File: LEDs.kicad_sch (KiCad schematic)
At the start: 26 parts, among them J3 JST-PH-1x3, J4 JST-PH-1x3, U4 SN74LVC1T45DBVR, U6 SN74LVC1T45DBVR

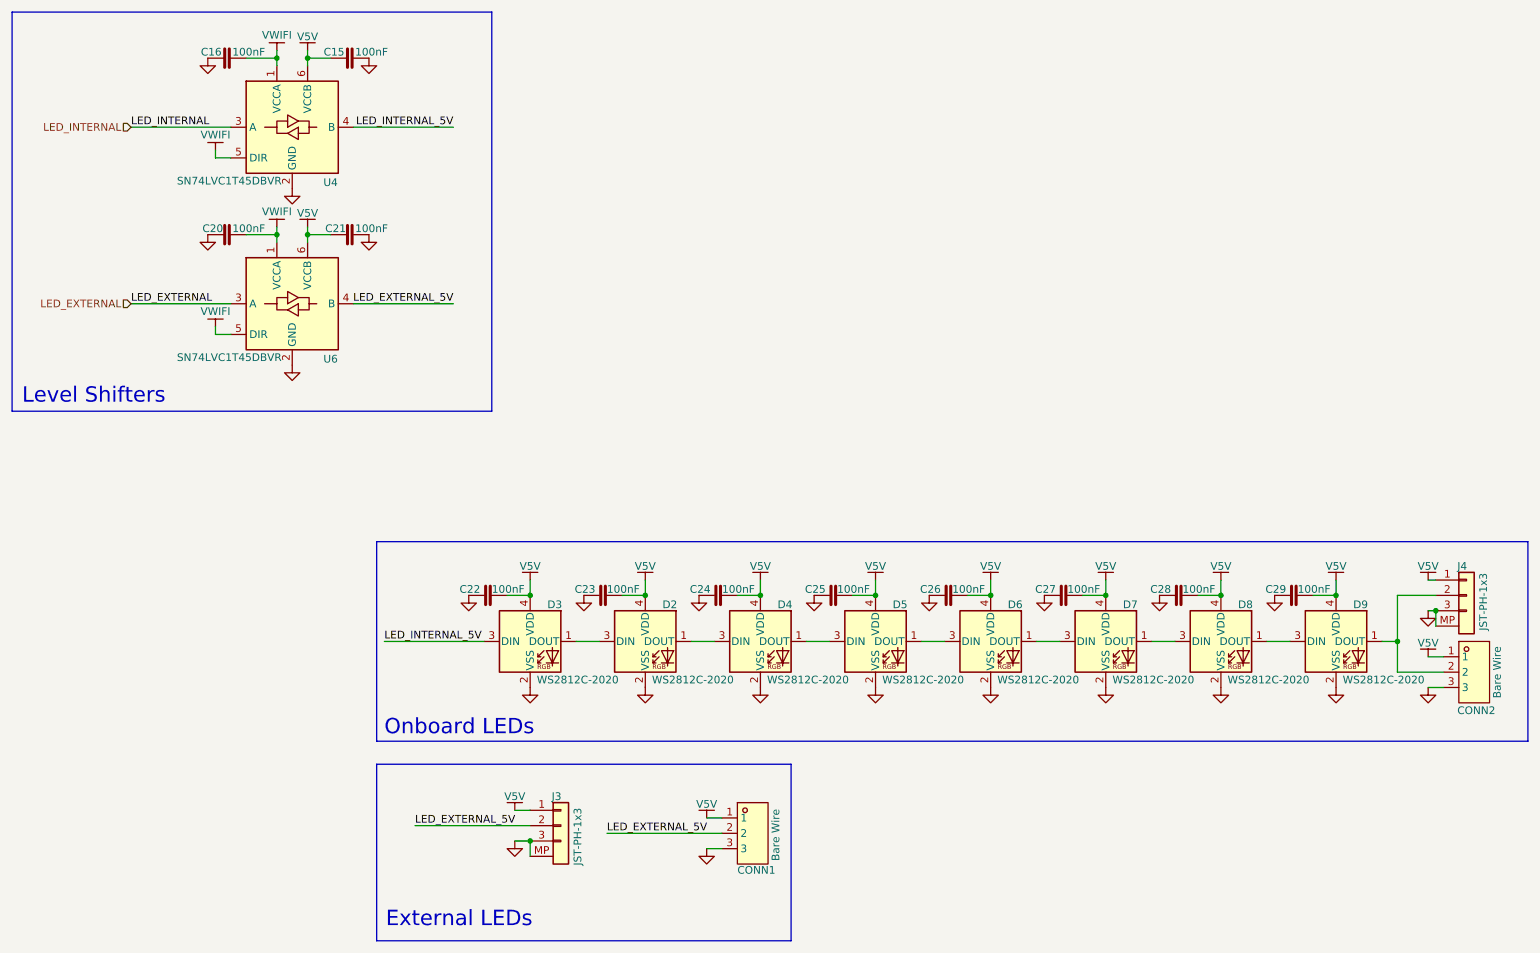
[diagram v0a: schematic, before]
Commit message: release evt2
Signed-off-by: Sean Cross <sean@xobs.io>
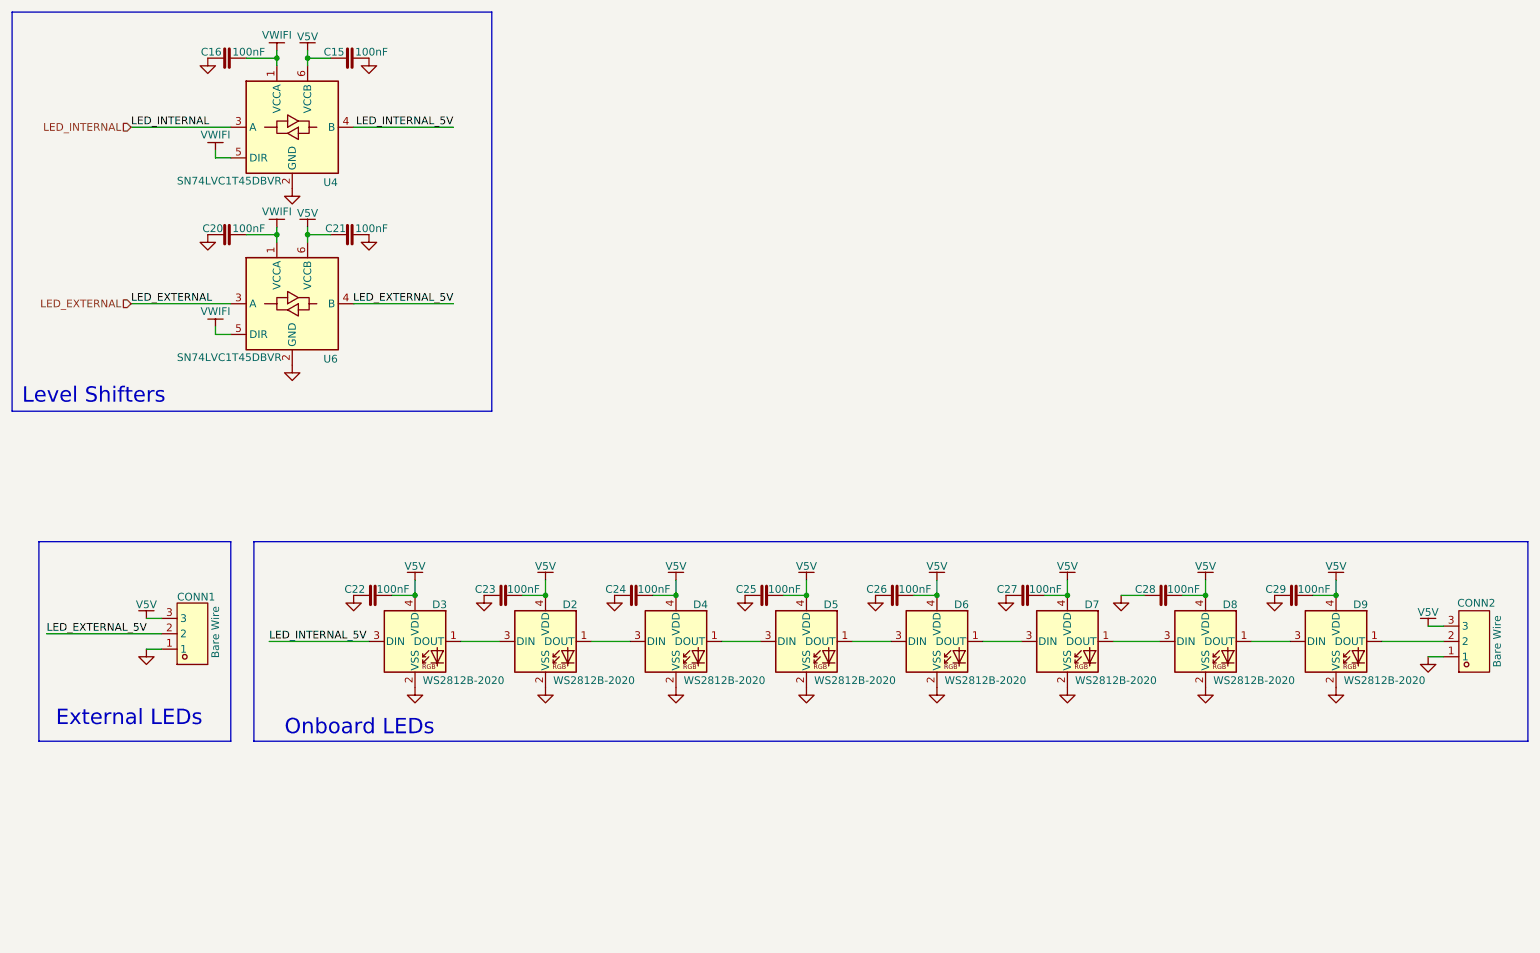
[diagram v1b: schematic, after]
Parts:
- removed J3, J4: JST-PH-1x3, Connector_JST:JST_PH_S3B-PH-SM4-TB_1x03-1MP_P2.00mm_Horizontal, symbol Galvani:JST-PH-2.0-1x3
- D2, D3, D4, D5, D6, D7, D8, D9: value WS2812C-2020 -> WS2812B-2020; symbol Galvani:WS2812C-2020 -> Galvani:WS2812B-2020; LCSC C2976072 -> C965555
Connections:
- net GND: now also CONN1.1, CONN2.1; no longer CONN1.3, CONN2.3
- net V5V: now also CONN1.3, CONN2.3; no longer CONN1.1, CONN2.1
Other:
- moved on the sheet: C22, C23, C24, C25, C26, C27, C28, CONN1, CONN2, D2, D3, D4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
